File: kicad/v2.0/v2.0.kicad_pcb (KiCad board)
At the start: 2 copper layers, 62.7 x 75.2 mm, 46 parts, among them J1 USB_B_Micro, J2 9V_IN, J3 MOTOR, J4 LED, J5 BUTTON, Q1 IRF520, SW1 RESET, SW2 FLASH, U1 MCP2221AxSL, U2 ZXBM5210-SP, U3 ESP32-WROOM-32, U4 AZ1117-3.3

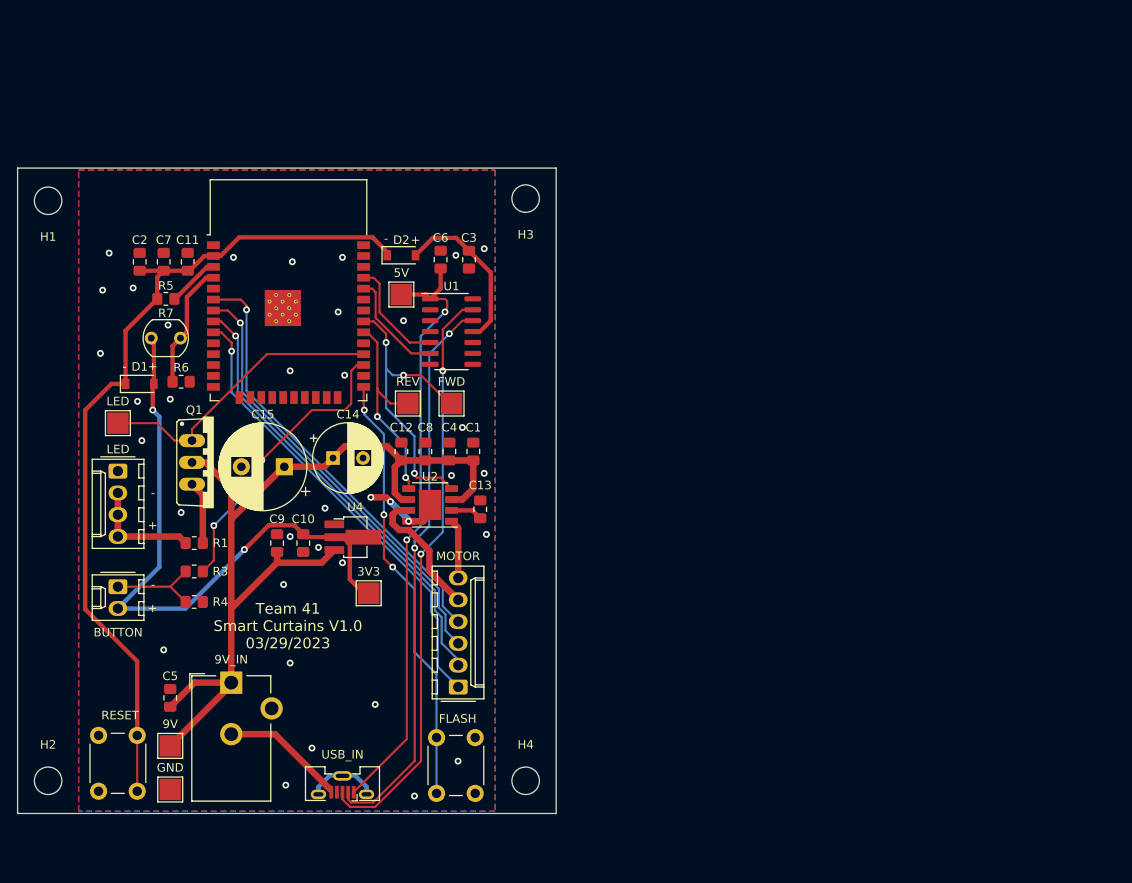
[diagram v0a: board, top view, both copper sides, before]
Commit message: v2.0 is done
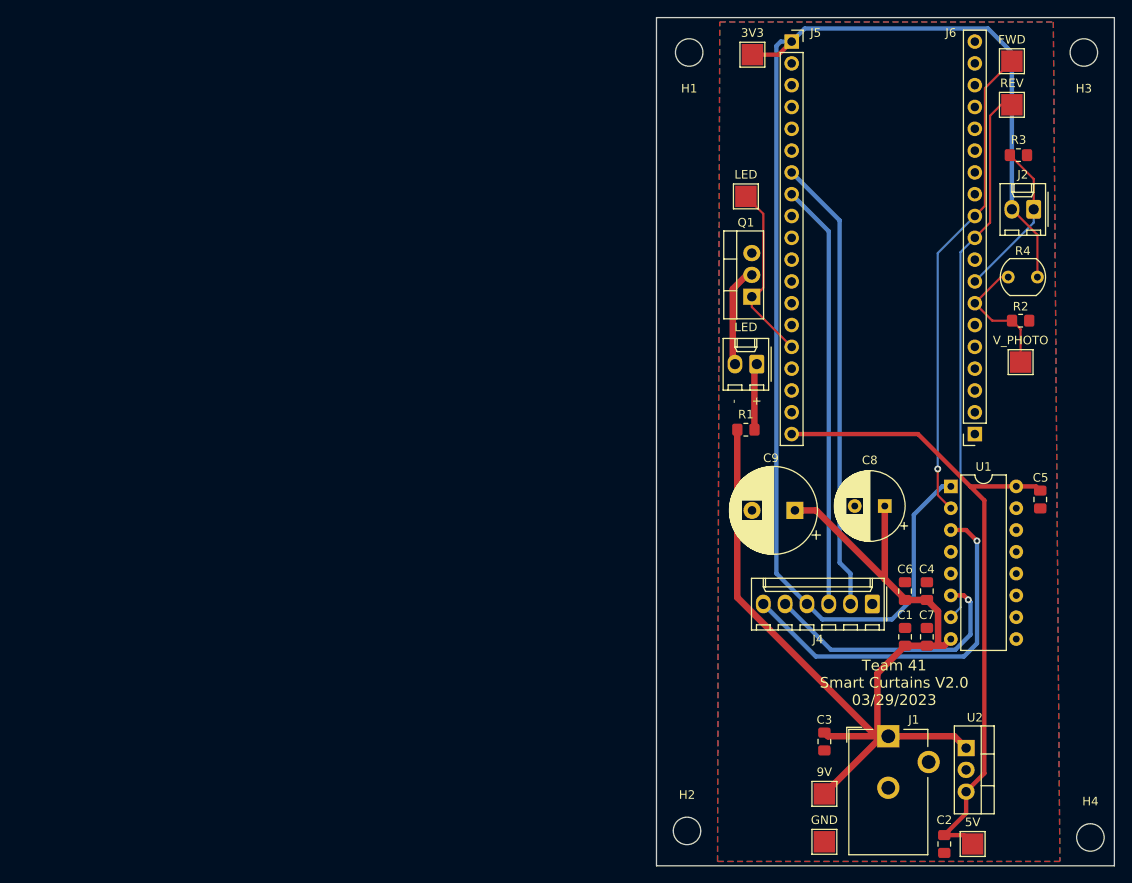
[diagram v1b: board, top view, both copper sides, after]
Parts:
- removed C10, C11, C12, C13: 22u, Capacitor_SMD:C_0805_2012Metric_Pad1.18x1.45mm_HandSolder
- removed C14: 220u, Capacitor_THT:CP_Radial_D8.0mm_P3.50mm
- removed C15: 470u, Capacitor_THT:CP_Radial_D10.0mm_P5.00mm
- removed D1, D2: MBR0520, Diode_SMD:D_SOD-123
- removed R5: 10k, Resistor_SMD:R_0805_2012Metric_Pad1.20x1.40mm_HandSolder
- removed R6: 20k, Resistor_SMD:R_0805_2012Metric_Pad1.20x1.40mm_HandSolder
- removed R7: R_Photo, OptoDevice:R_LDR_5.1x4.3mm_P3.4mm_Vertical
- removed SW1: RESET, Button_Switch_THT:SW_PUSH_6mm
- removed SW2: FLASH, Button_Switch_THT:SW_PUSH_6mm
- removed U3: ESP32-WROOM-32, RF_Module:ESP32-WROOM-32
- removed U4: AZ1117-3.3, Package_TO_SOT_SMD:SOT-89-3_Handsoldering
- added J6: DEV BOARD RIGHT, Connector_PinSocket_2.54mm:PinSocket_1x19_P2.54mm_Vertical, F.Cu at (225.3, 81.3)
- added R2: 3.3k, Resistor_SMD:R_0805_2012Metric_Pad1.20x1.40mm_HandSolder, F.Cu at (230.6, 68.1)
- added TP8: V_PHOTO, TestPoint:TestPoint_Pad_2.5x2.5mm, F.Cu at (230.6, 72.9)
- C1, C2: value .1u -> 0.1u
- C3: value .47u -> 0.33u
- C7: value 1u -> 10u
- C8: value 10u -> 220u; footprint Capacitor_SMD:C_0805_2012Metric_Pad1.18x1.45mm_HandSolder -> Capacitor_THT:CP_Radial_D8.0mm_P3.50mm
- C9: value 10u -> 470u; footprint Capacitor_SMD:C_0805_2012Metric_Pad1.18x1.45mm_HandSolder -> Capacitor_THT:CP_Radial_D10.0mm_P5.00mm
- J1: value USB_B_Micro -> 9V_IN; footprint Connector_USB:USB_Micro-B_Molex-105133-0031 -> Connector_BarrelJack:BarrelJack_CUI_PJ-102AH_Horizontal
- J2: value 9V_IN -> BUTTON; footprint Connector_BarrelJack:BarrelJack_CUI_PJ-102AH_Horizontal -> Connector_Molex:Molex_KK-254_AE-6410-02A_1x02_P2.54mm_Vertical
- J3: value MOTOR -> LED STRIP; footprint Connector_Molex:Molex_KK-254_AE-6410-06A_1x06_P2.54mm_Vertical -> Connector_Molex:Molex_KK-254_AE-6410-02A_1x02_P2.54mm_Vertical
- J4: value LED -> MOTOR; footprint Connector_Molex:Molex_KK-254_AE-6410-04A_1x04_P2.54mm_Vertical -> Connector_Molex:Molex_KK-254_AE-6410-06A_1x06_P2.54mm_Vertical
- J5: value BUTTON -> DEV BOARD LEFT; footprint Connector_Molex:Molex_KK-254_AE-6410-02A_1x02_P2.54mm_Vertical -> Connector_PinSocket_2.54mm:PinSocket_1x19_P2.54mm_Vertical
- Q1: value IRF520 -> FQP30N06L; footprint IRF520:TO220BV -> Package_TO_SOT_THT:TO-220-3_Vertical
- R1: value 1k -> 100
- R3: value 1k -> 10k
- R4: value 1k -> R_Photo; footprint Resistor_SMD:R_0805_2012Metric_Pad1.20x1.40mm_HandSolder -> OptoDevice:R_LDR_5.1x4.3mm_P3.4mm_Vertical
- TP1: value LED -> GND
- TP2: value FWD -> 9V
- TP3: value REV -> 5V
- TP4: value 9V -> 3V3
- TP5: value 3V3 -> FWD
- TP6: value 5V -> REV
- TP7: value GND -> LED
- U1: value MCP2221AxSL -> L293D; footprint Package_SO:SOIC-14_3.9x8.7mm_P1.27mm -> Package_DIP:DIP-16_W7.62mm
- U2: value ZXBM5210-SP -> L7805; footprint Package_SO:Diodes_SO-8EP -> Package_TO_SOT_THT:TO-220-3_Vertical
- moved C2 115.7 mm to (221.7, 129.0), turned to -90 degrees
- moved J2 108.5 mm to (232.2, 55.1), turned to 180 degrees
- moved R3 107.6 mm to (230.4, 48.8)
- moved TP4 105.3 mm to (199.4, 37.1)
- moved R4 105.3 mm to (232.6, 63.0), turned to 180 degrees
- moved C5 103.9 mm to (232.9, 88.9)
- moved J5 101.0 mm to (204.0, 35.6), turned to 0 degrees
- moved C7 99.1 mm to (219.7, 104.9)
- moved TP5 97.2 mm to (229.6, 37.8)
- moved TP7 96.3 mm to (198.6, 53.6)
- moved TP1 95.7 mm to (207.8, 128.8)
- moved J4 89.2 mm to (213.4, 101.1), turned to 180 degrees
- moved TP3 83.4 mm to (225.0, 129.0)
- moved H1 76.6 mm to (192.0, 36.8)
- moved H2 74.7 mm to (191.8, 127.5)
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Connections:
- C2 pad 1: Net-(C11-Pad1) -> +5V
- C3 pad 1: /3V3_USB -> +9V
- C5 pad 1: +9V -> GND
- C5 pad 2: GND -> +5V
- C6 pad 1: Net-(C6-Pad1) -> +9V
- C7 pad 1: Net-(C11-Pad1) -> +9V
- J1 pad 1: Net-(C6-Pad1) -> +9V
- J1 pad 2: Net-(J1-Pad2) -> GND
- J1 pad 3: Net-(J1-Pad3) -> (no net)
- J2 pad 1: +9V -> Net-(R3-Pad1)
- J2 pad 2: GND -> +3V3
- J3 pad 1: /GPIO34 -> Net-(J3-Pad1)
- J3 pad 2: /GPIO35 -> Net-(J3-Pad2)
- J4 pad 2: Net-(J4-Pad2) -> /ENCODER2
- J4 pad 3: Net-(J4-Pad2) -> /ENCODER1
- J4 pad 4: Net-(J4-Pad2) -> +3V3
- J5 pad 1: Net-(J5-Pad1) -> +3V3
- J5 pad 2: /3V3_INPUT -> unconnected-(J5-Pad2)
- R1 pad 1: Net-(Q1-PadS) -> +9V
- R1 pad 2: Net-(J4-Pad2) -> Net-(J3-Pad1)
- R3 pad 1: Net-(J5-Pad1) -> Net-(R3-Pad1)
- R3 pad 2: Net-(R3-Pad2) -> GND
- R4 pad 1: Net-(J5-Pad1) -> +3V3
- R4 pad 2: GND -> /V_PHOTO
- TP1 pad 1: /LED -> GND
- TP2 pad 1: /FWD -> +9V
- TP3 pad 1: /REV -> +5V
- TP4 pad 1: +9V -> +3V3
- TP5 pad 1: /3V3_INPUT -> /FWD
- TP6 pad 1: Net-(C6-Pad1) -> /REV
- TP7 pad 1: GND -> /LED
- U1 pad 1: Net-(C6-Pad1) -> +3V3
- U1 pad 11: /3V3_USB -> unconnected-(U1-Pad11)
- U1 pad 12: Net-(J1-Pad2) -> GND
- U1 pad 13: Net-(J1-Pad3) -> GND
- U1 pad 14: GND -> unconnected-(U1-Pad14)
- U1 pad 2: unconnected-(U1-Pad2) -> /FWD
- U1 pad 3: unconnected-(U1-Pad3) -> Net-(J4-Pad6)
- U1 pad 4: unconnected-(U1-Pad4) -> GND
- U1 pad 5: /TXD0 -> GND
- U1 pad 6: /RXD0 -> Net-(J4-Pad5)
- U1 pad 7: unconnected-(U1-Pad7) -> /REV
- U1 pad 8: unconnected-(U1-Pad8) -> +9V
- U2 pad 1: Net-(J3-Pad6) -> +9V
- U2 pad 2: Net-(C13-Pad1) -> GND
- U2 pad 3: +9V -> +5V
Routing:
- net +3V3: track 0.00 -> 158.1 mm
- net Net-(C11-Pad1): track 99.4 -> 0.00 mm
- net +5V: track 0.00 -> 78.6 mm
- net /3V3_INPUT: track 74.4 -> 0.00 mm, vias 2 -> 0
- net Net-(C6-Pad1): track 71.4 -> 0.00 mm, vias 2 -> 0
- net Net-(J1-Pad3): track 68.3 -> 0.00 mm, vias 2 -> 0
- net Net-(J1-Pad2): track 65.6 -> 0.00 mm, vias 2 -> 0
- net /GPIO34: track 53.7 -> 0.00 mm, vias 1 -> 0
- net /ENCODER2: track 0.00 -> 53.1 mm
- net /GPIO35: track 52.4 -> 0.00 mm, vias 1 -> 0
- net /GPIO32: track 51.6 -> 0.00 mm, vias 1 -> 0
- net /GPIO33: track 51.2 -> 0.00 mm, vias 1 -> 0
- net Net-(SW2-Pad1): track 50.9 -> 0.00 mm, vias 3 -> 0
- net /ENCODER1: track 0.00 -> 49.5 mm
- net Net-(J4-Pad6): track 0.00 -> 43.6 mm, vias 0 -> 1
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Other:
- board size 62.7 x 75.2 mm -> 53.3 x 98.8 mm
- board text added: "Team 41 Smart Curtains V2.0 03/29/2023"
- board text removed: "Team 41 Smart Curtains V1.0 03/29/2023"
